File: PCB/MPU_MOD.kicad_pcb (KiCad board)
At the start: 8 copper layers, 43.5 x 70 mm, 305 parts, among them J1 SJ-43504-SMT-TR, J2 2-1734248-0, J3 USB4510-03-1-A_REVA, J501 MEM2090-00-145-00-A_REVA, J701 FTSH-107-01-L-DV-K-A, J901 73412-0110, U1 IS21ES08GA-JQLI-TR, U201 STC3115IQT, U203 STPMIC1APQR, U3 BQ24298RTWR, U301 STM32MP157FABx, U401 MT41K256M16TW-107_P, U502 HSP051-4M10, U503 HSP051-4M10, U701 HSP051-4M10, U702 HSP051-4M10, U801 FUSB302BMPX, U802 HSP051-4M10, U901 LBEE5PK2AE-771, Y601 NX2012SA-32.768K, Y701 ECS-2520MVQ-240

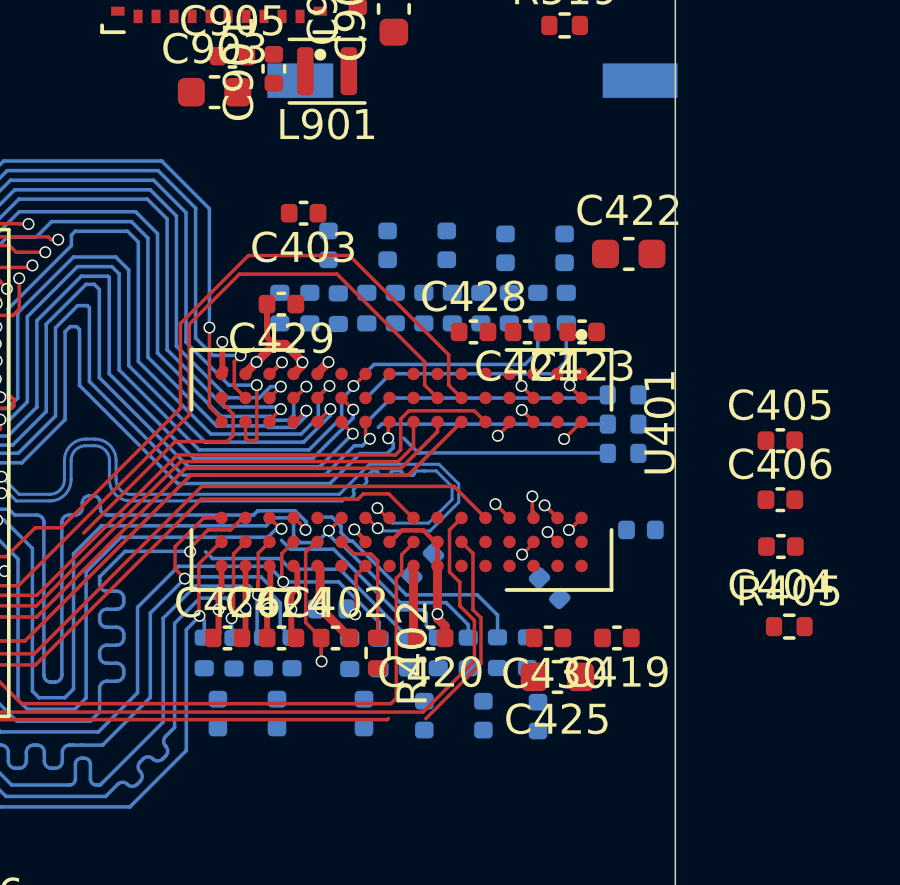
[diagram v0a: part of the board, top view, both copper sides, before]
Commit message: PCB_UPDATE
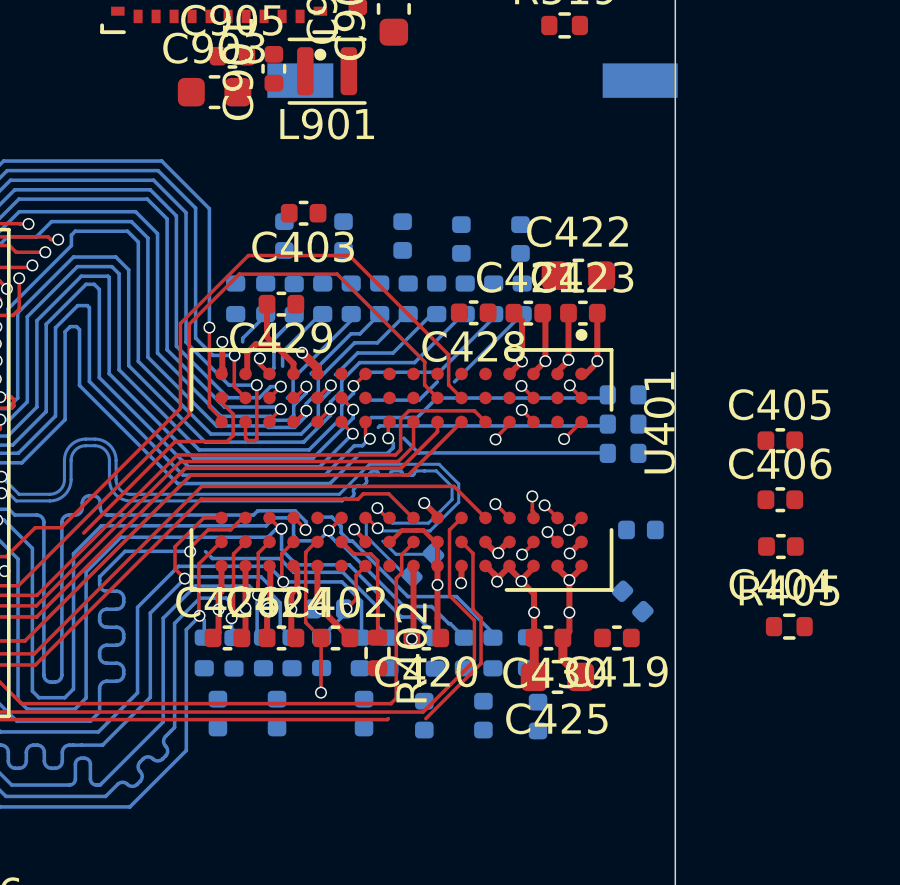
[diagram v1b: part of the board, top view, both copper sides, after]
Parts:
- moved C427 2.80 mm to (110.6, 73.2)
- moved R419 2.49 mm to (97.3, 63.1)
- moved C422 1.83 mm to (108.8, 62.3)
- moved R415 1.50 mm to (99.3, 63.1)
- moved R421 1.50 mm to (104.0, 63.1)
- moved C409 1.50 mm to (99.0, 61.0)
- moved C410 1.50 mm to (100.9, 61.0)
- moved C411 1.50 mm to (102.9, 61.0)
- moved C413 1.50 mm to (106.8, 61.1)
- moved C414 1.50 mm to (104.9, 61.1)
- moved R406 1.50 mm to (103.1, 63.1)
- moved R408 1.50 mm to (101.2, 63.1)
- moved R409 1.50 mm to (102.1, 63.1)
- moved R411 1.50 mm to (100.2, 63.1)
- moved R423 1.50 mm to (105.0, 63.1)
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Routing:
- net VDD_DDR: track 21.4 -> 33.5 mm, vias 19 -> 25
- net GND: track 77.6 -> 88.9 mm, vias 96 -> 102
- net /DDR/DDR_BA2: track 24.0 -> 30.1 mm
- net /DDR/DDR_A0: track 24.2 -> 29.3 mm
- net /DDR/DDR_BA0: track 23.9 -> 28.1 mm
- net /DDR/DDR_A2: track 23.6 -> 27.3 mm
- net /DDR/DDR_A9: track 25.2 -> 28.4 mm
- net /DDR/DDR_A3: track 23.3 -> 26.4 mm
- net /DDR/DDR_CLK_P: track 23.8 -> 26.5 mm
- net /DDR/DDR_CSN: track 32.4 -> 29.7 mm
- net /DDR/DDR_A5: track 25.4 -> 27.8 mm
- net /DDR/DDR_ODT: track 30.0 -> 28.1 mm
- net /DDR/DDR_CLK_N: track 23.9 -> 25.7 mm
- net /DDR/DDR_CKE: track 19.8 -> 21.0 mm
- net VREF_DDR: track 6.21 -> 7.25 mm
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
